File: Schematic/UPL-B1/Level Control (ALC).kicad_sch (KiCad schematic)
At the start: 102 parts, among them P53 TestPoint, P54 TestPoint, P55 TestPoint, P56 TestPoint, P57 TestPoint, P58 TestPoint, X50 Conn_01x03_Pin_Bridge, X51 Conn_01x03_Pin_Bridge, X52 Conn_01x03_Pin_Bridge

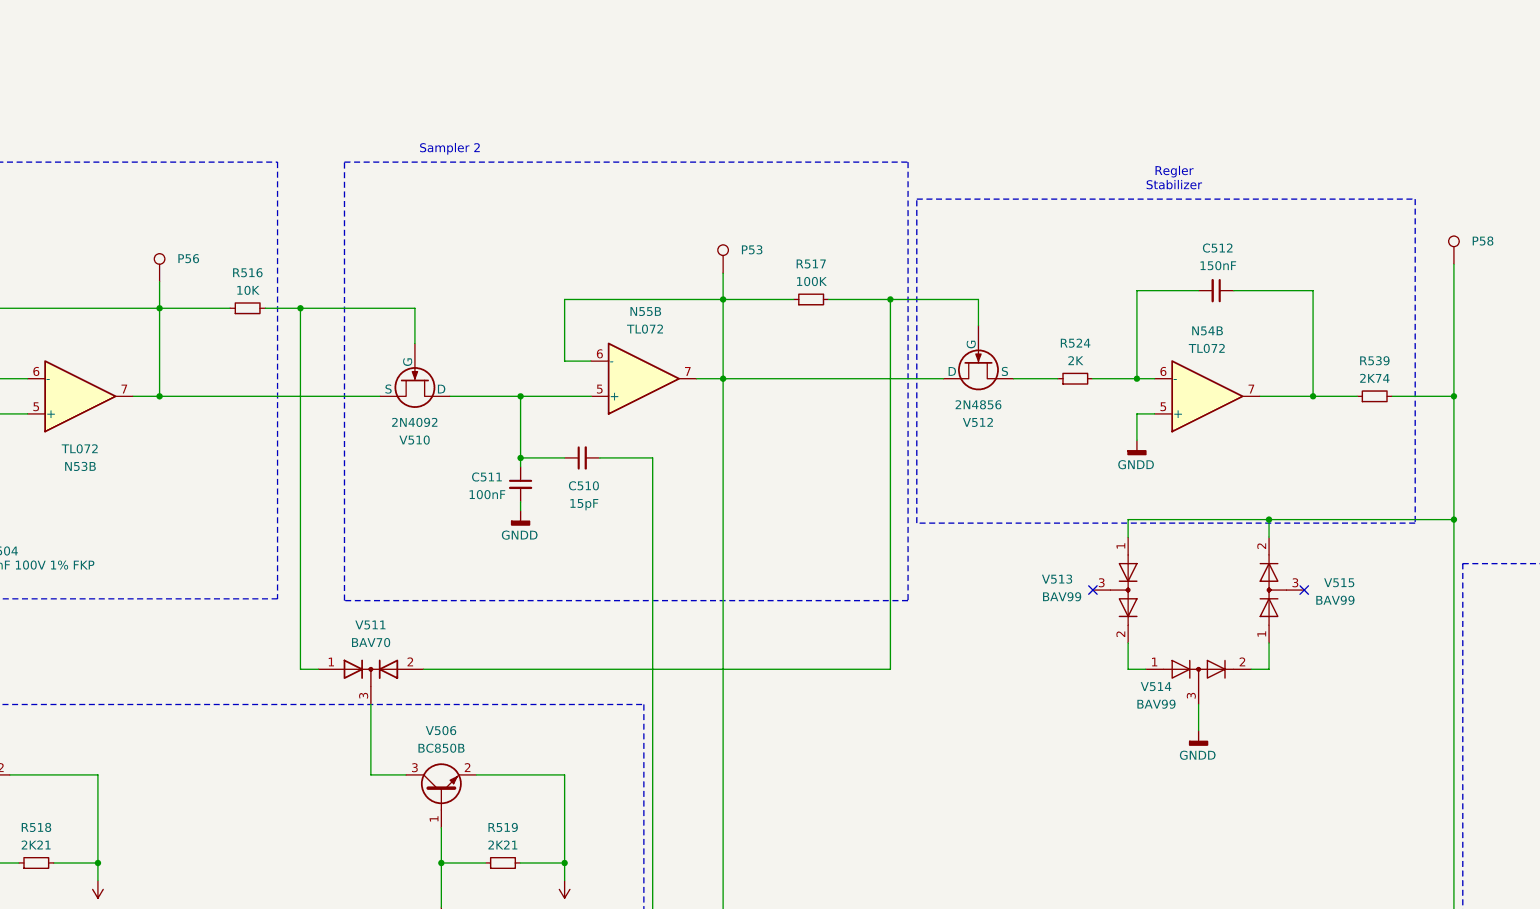
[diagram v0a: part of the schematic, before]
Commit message: Some visual cleanup
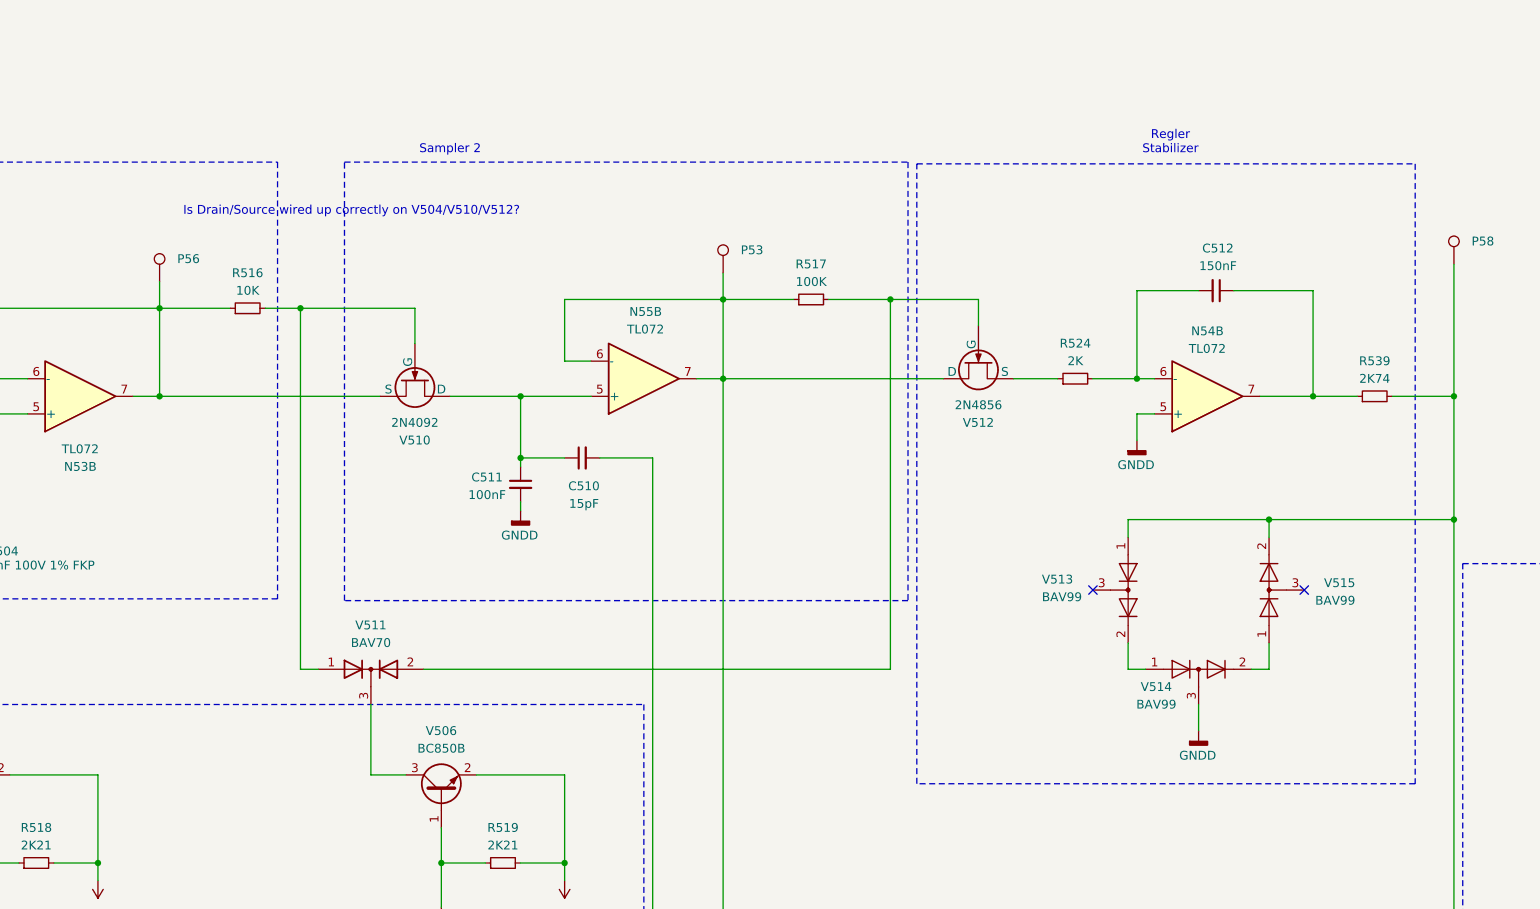
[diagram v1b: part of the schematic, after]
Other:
- note added: "Is Drain/Source wired up correctly on V504/V510/V512?"
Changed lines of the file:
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@@
 	)
 	(rectangle
-		(start 327.66 115.062)
-		(end 399.542 161.798)
+		(start 327.66 109.982)
+		(end 399.542 199.39)
 		(stroke
 			(width 0)
@@
 	(text "Regler\nStabilizer"
 		(exclude_from_sim no)
-		(at 364.744 112.268 0)
+		(at 364.236 106.934 0)
 		(effects
 			(font
@@
 			)
 		)
+	)
+	(text "Is Drain/Source wired up correctly on V504/V510/V512?"
+		(exclude_from_sim no)
+		(at 246.126 116.84 0)
+		(effects
+			(font
+				(size 1.27 1.27)
+				(color 255 0 43 1)
+			)
+		)
